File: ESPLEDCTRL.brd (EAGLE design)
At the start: 70.2 x 30.2 mm, 15 parts, among them IC1 74HC1G08GW

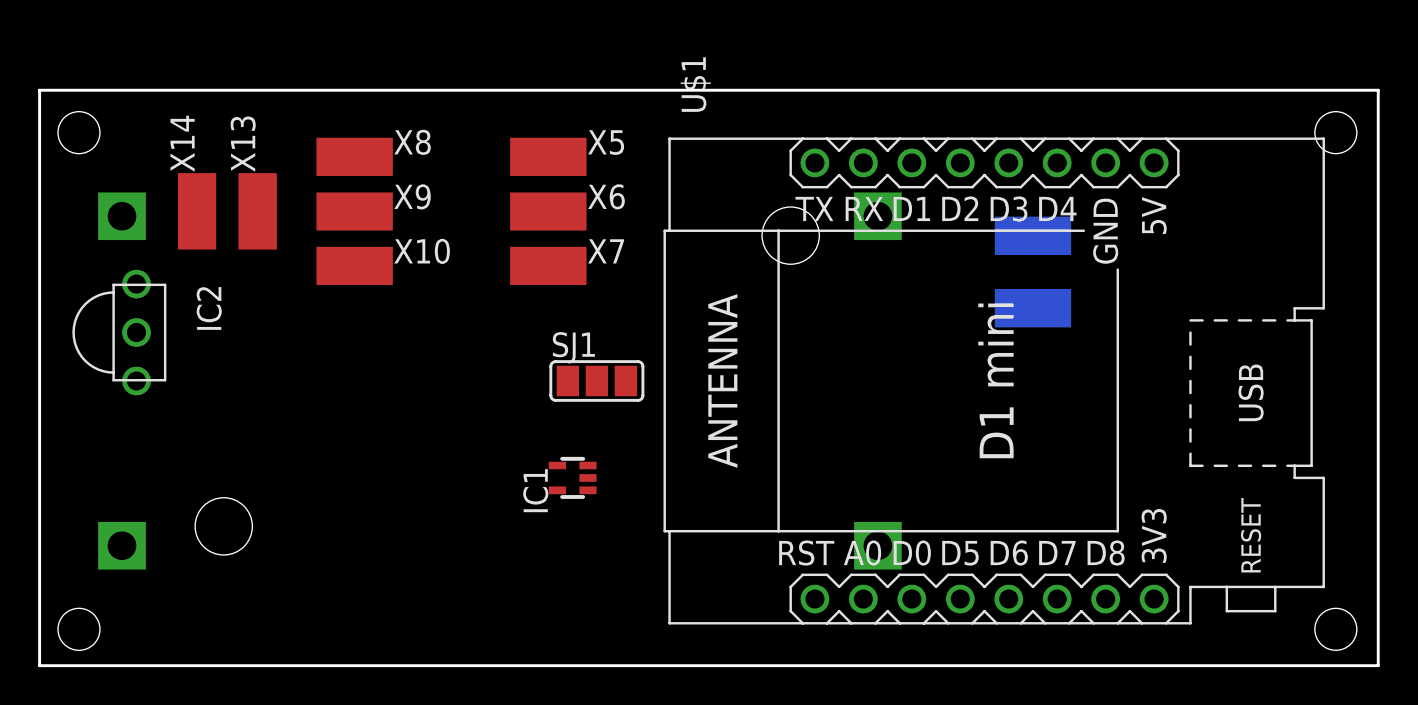
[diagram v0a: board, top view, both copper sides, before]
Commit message: Board fertig gestellt
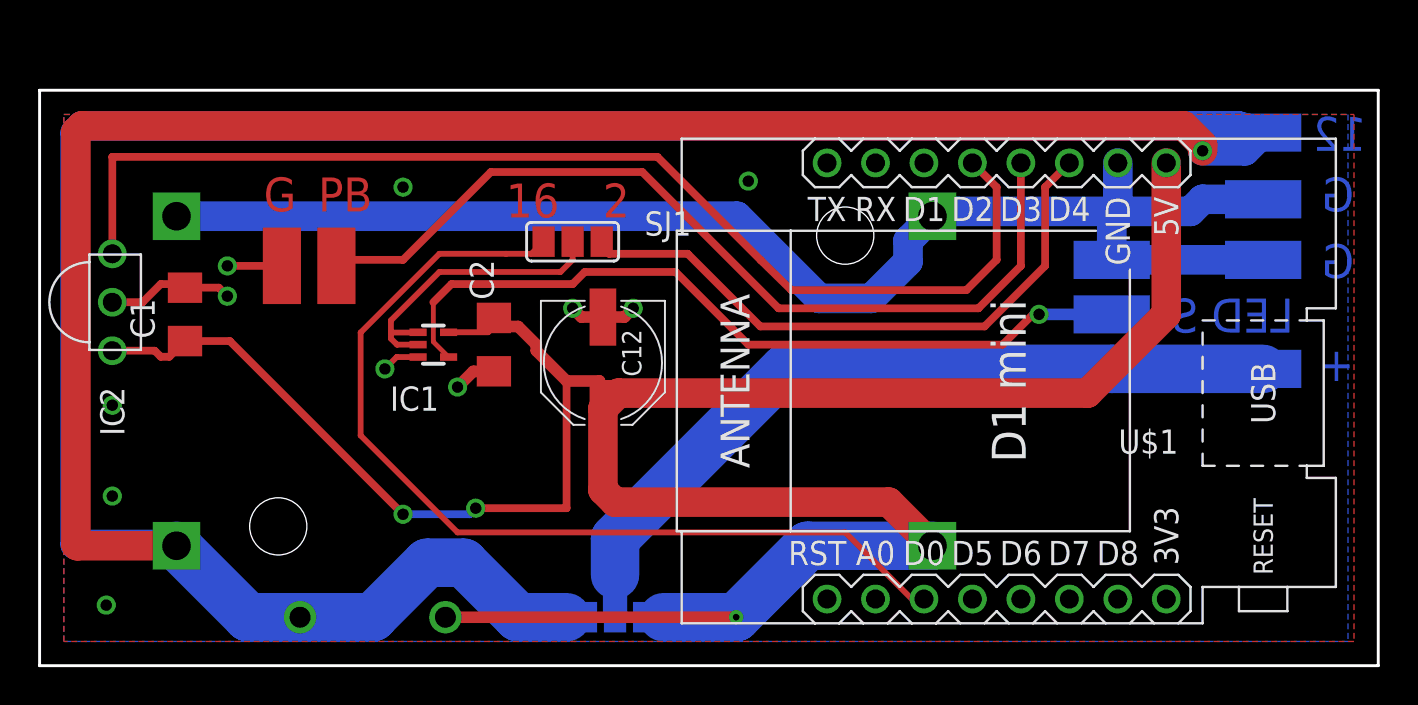
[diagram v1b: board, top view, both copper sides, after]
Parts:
- removed X9: (no value), modules:PAD2X4
- added C1, C2: (no value), rcl:C1206
- added C12: 100uF, rcl:PANASONIC_D
- added D1: 1N5819-T, diode:DO41-7.6
- added SJ2: (no value), jumper:SJ_2
- moved X8 48.9 mm to (59.1, 10.8), flipped to the bottom
- moved X10 47.6 mm to (59.1, 16.5), flipped to the bottom
- moved X5 31.5 mm to (51.1, 10.8), flipped to the bottom
- moved X6 30.0 mm to (51.1, 13.7), flipped to the bottom
- moved X7 29.5 mm to (51.1, 16.5), flipped to the bottom
- moved X12 13.4 mm to (59.1, 19.7)
- moved X11 13.2 mm to (59.1, 23.2)
- moved IC1 10.1 mm to (15.6, 12.1), turned to 270 degrees
- moved SJ1 7.41 mm to (22.9, 17.5), turned to 180 degrees
- moved X14 5.28 mm to (7.62, 16.2)
- moved X13 5.02 mm to (10.5, 16.2)
- moved U$2 2.86 mm to (21.9, 10.2)
- moved IC2 2.03 mm to (-1.27, 14.3)
- moved U$1 0.63 mm to (45.7, 10.2)
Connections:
- removed net N$21: U$2.IN+, X11.P$1
- new net +12V: D1.C, SJ2.1, U$2.IN+, X11.P$1
- new net V+: SJ2.2, X5.P$1, X8.P$1
- net +5V: now also C1.1, C12.+, C2.1, D1.A, SJ2.3; no longer X5.P$1, X8.P$1
- net GND: now also C1.2, C12.-, C2.2
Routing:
- net +12V: track 0.00 -> 205.6 mm, vias 0 -> 1
- net +5V: track 0.00 -> 140.3 mm, vias 0 -> 3
- net GND: track 0.00 -> 92.0 mm, vias 0 -> 11
- net N$2: track 0.00 -> 60.6 mm
- net N$17: track 0.00 -> 50.0 mm
- net N$1: track 0.00 -> 47.2 mm
- net V+: track 0.00 -> 41.8 mm
- net N$18: track 0.00 -> 41.7 mm, vias 0 -> 1
- net N$15: track 0.00 -> 32.4 mm
- net N$16: track 0.00 -> 15.7 mm
- added copper zone on layer 1, net GND
- added copper zone on layer 16, net GND
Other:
- board text added: "+"
- board text added: "12"
- board text added: "16"
- board text added: "2"
- board text added: "5"
- board text added: "G"
- board text added: "LED S"
- board text added: "PB"
